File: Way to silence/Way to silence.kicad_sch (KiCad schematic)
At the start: 17 parts, among them J3 5V_Terminal, J4 Battery_Terminal, J5 LEDS Port, SW1 SW_SPDT, SW3 SW_SPST, U1 ESP32-WROOM-32-N16, U6 AMS1117CD-3.3

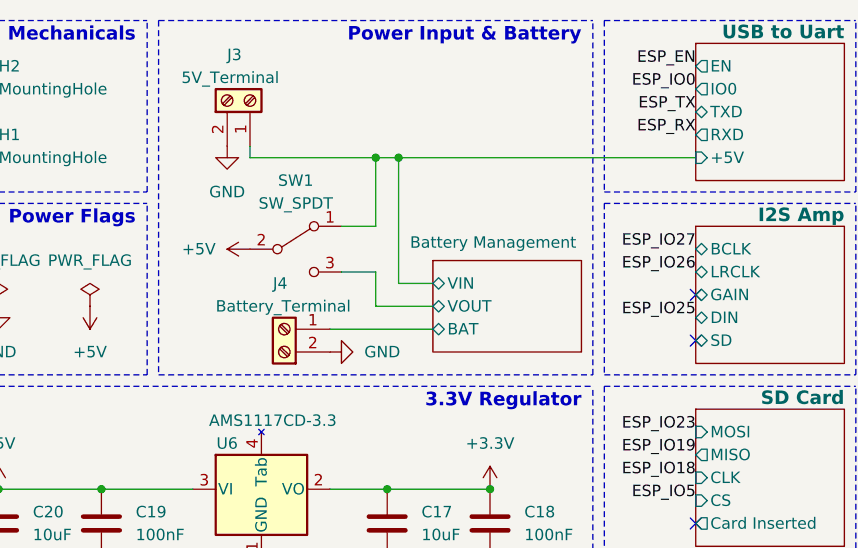
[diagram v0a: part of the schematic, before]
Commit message: [UDPT] Sheet name
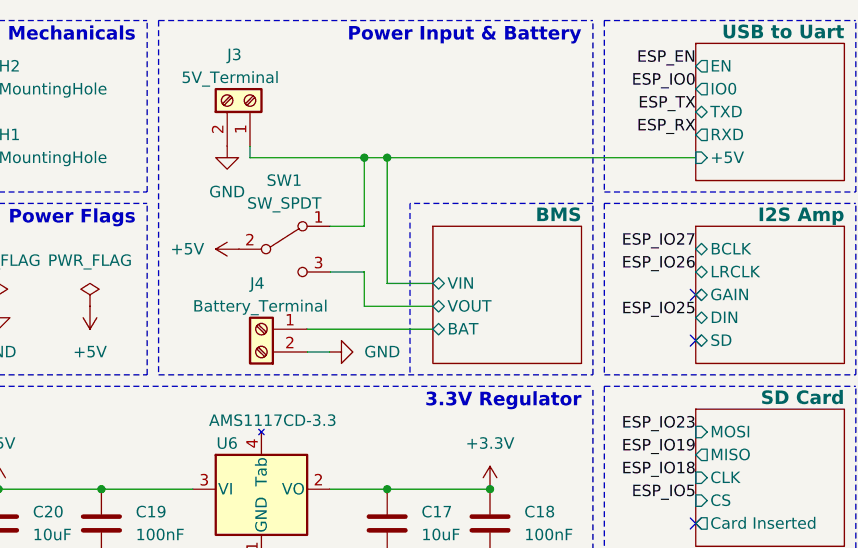
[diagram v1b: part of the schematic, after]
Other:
- sheet Battery Management renamed BMS
- moved on the sheet: J4, SW1
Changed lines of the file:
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@@
     (rev "1.0")
   )
-  (junction (at 144.78 30.48) (diameter 0) (color 0 0 0 0)
-  )
-  (junction (at 142.24 30.48) (diameter 0) (color 0 0 0 0)
-  )
   (junction (at 143.51 67.31) (diameter 0) (color 0 0 0 0)
   )
   (junction (at 100.33 67.31) (diameter 0) (color 0 0 0 0)
   )
+  (junction (at 143.51 30.48) (diameter 0) (color 0 0 0 0)
+  )
   (junction (at 111.76 67.31) (diameter 0) (color 0 0 0 0)
   )
   (junction (at 154.94 67.31) (diameter 0) (color 0 0 0 0)
+  )
+  (junction (at 140.97 30.48) (diameter 0) (color 0 0 0 0)
   )
   (junction (at 154.94 74.93) (diameter 0) (color 0 0 0 0)
@@
     (stroke (width 0) (type dash))
   )
-  (wire (pts (xy 148.59 46.99) (xy 142.24 46.99))
+  (wire (pts (xy 143.51 30.48) (xy 177.8 30.48))
+    (stroke (width 0) (type default))
+  )
+  (wire (pts (xy 148.59 46.99) (xy 140.97 46.99))
     (stroke (width 0) (type default))
   )
@@
     (stroke (width 0) (type dash))
   )
-  (wire (pts (xy 138.43 38.1) (xy 142.24 38.1))
+  (wire (pts (xy 137.16 38.1) (xy 140.97 38.1))
     (stroke (width 0) (type default))
   )
@@
     (stroke (width 0) (type dash))
   )
-  (wire (pts (xy 142.24 30.48) (xy 128.27 30.48))
+  (wire (pts (xy 140.97 30.48) (xy 143.51 30.48))
     (stroke (width 0) (type default))
   )
@@
     (stroke (width 0) (type dash))
   )
-  (wire (pts (xy 144.78 44.45) (xy 148.59 44.45))
+  (wire (pts (xy 143.51 44.45) (xy 148.59 44.45))
     (stroke (width 0) (type default))
   )
@@
     (stroke (width 0) (type dash))
   )
-  (wire (pts (xy 142.24 46.99) (xy 142.24 43.18))
+  (wire (pts (xy 140.97 46.99) (xy 140.97 43.18))
     (stroke (width 0) (type default))
   )
@@
     (stroke (width 0) (type dash))
   )
-  (wire (pts (xy 142.24 38.1) (xy 142.24 30.48))
+  (wire (pts (xy 140.97 38.1) (xy 140.97 30.48))
     (stroke (width 0) (type default))
   )
@@
     (stroke (width 0) (type dash))
   )
+  (polyline (pts (xy 166.37 35.56) (xy 146.05 35.56))
+    (stroke (width 0) (type dash))
+  )
   (wire (pts (xy 100.33 74.93) (xy 111.76 74.93))
     (stroke (width 0) (type default))
@@
     (stroke (width 0) (type dash))
   )
-  (wire (pts (xy 142.24 30.48) (xy 144.78 30.48))
-    (stroke (width 0) (type default))
-  )
   (polyline (pts (xy 60.96 15.24) (xy 60.96 34.29))
     (stroke (width 0) (type dash))
@@
     (stroke (width 0) (type dash))
   )
+  (wire (pts (xy 134.62 52.07) (xy 137.16 52.07))
+    (stroke (width 0) (type default))
+  )
   (polyline (pts (xy 167.64 74.93) (xy 195.58 74.93))
     (stroke (width 0) (type dash))
@@
     (stroke (width 0) (type dash))
   )
-  (wire (pts (xy 144.78 30.48) (xy 144.78 44.45))
+  (wire (pts (xy 143.51 30.48) (xy 143.51 44.45))
     (stroke (width 0) (type default))
   )
@@
     (stroke (width 0) (type dash))
   )
+  (polyline (pts (xy 146.05 35.56) (xy 146.05 54.61))
+    (stroke (width 0) (type dash))
+  )
   (polyline (pts (xy 195.58 74.93) (xy 195.58 55.88))
     (stroke (width 0) (type dash))
@@
     (stroke (width 0) (type dash))
   )
-  (wire (pts (xy 137.16 49.53) (xy 148.59 49.53))
+  (wire (pts (xy 134.62 49.53) (xy 148.59 49.53))
     (stroke (width 0) (type default))
   )
@@
     (stroke (width 0) (type default))
   )
+  (wire (pts (xy 140.97 30.48) (xy 128.27 30.48))
+    (stroke (width 0) (type default))
+  )
   (polyline (pts (xy 92.71 34.29) (xy 92.71 15.24))
     (stroke (width 0) (type dash))
@@
     (stroke (width 0) (type dash))
   )
-  (wire (pts (xy 144.78 30.48) (xy 177.8 30.48))
-    (stroke (width 0) (type default))
-  )
   (polyline (pts (xy 93.98 82.55) (xy 166.37 82.55))
     (stroke (width 0) (type dash))
@@
     (stroke (width 0) (type dash))
   )
-  (wire (pts (xy 142.24 43.18) (xy 138.43 43.18))
+  (wire (pts (xy 140.97 43.18) (xy 137.16 43.18))
     (stroke (width 0) (type default))
   )
@@
     )
   )
-  (symbol (lib_id "power:+5V") (at 128.27 40.64 90) (unit 1)
-    (in_bom yes) (on_board yes) (dnp no) (fields_autoplaced)
-    (property "Reference" "#PWR06" (at 132.08 40.64 0)
-      (effects (font (size 1.27 1.27)) hide)
-    )
-    (property "Value" "+5V" (at 124.46 40.64 90)
-      (effects (font (size 1.27 1.27)) (justify left))
-    )
-    (property "Footprint" "" (at 128.27 40.64 0)
-      (effects (font (size 1.27 1.27)) hide)
-    )
-    (property "Datasheet" "" (at 128.27 40.64 0)
+  (symbol (lib_id "power:+5V") (at 127 40.64 90) (unit 1)
+    (in_bom yes) (on_board yes) (dnp no) (fields_autoplaced)
+    (property "Reference" "#PWR06" (at 130.81 40.64 0)
+      (effects (font (size 1.27 1.27)) hide)
+    )
+    (property "Value" "+5V" (at 123.19 40.64 90)
+      (effects (font (size 1.27 1.27)) (justify left))
+    )
+    (property "Footprint" "" (at 127 40.64 0)
+      (effects (font (size 1.27 1.27)) hide)
+    )
+    (property "Datasheet" "" (at 127 40.64 0)
       (effects (font (size 1.27 1.27)) hide)
     )
@@
     )
   )
-  (symbol (lib_id "Way to silence:SW_SPDT") (at 133.35 40.64 0) (unit 1)
-    (in_bom yes) (on_board yes) (dnp no) (fields_autoplaced)
-    (property "Reference" "SW1" (at 133.35 33.02 0)
-      (effects (font (size 1.27 1.27)))
-    )
-    (property "Value" "SW_SPDT" (at 133.35 35.56 0)
-      (effects (font (size 1.27 1.27)))
-    )
-    (property "Footprint" "Way to silence:SW_SPDT" (at 132.08 26.67 0)
-      (effects (font (size 1.27 1.27)) hide)
-    )
-    (property "Datasheet" "~" (at 133.35 29.21 0)
-      (effects (font (size 1.27 1.27)) hide)
-    )
-    (property "LCSC" "C319013" (at 132.08 24.13 0)
+  (symbol (lib_id "Way to silence:SW_SPDT") (at 132.08 40.64 0) (unit 1)
+    (in_bom yes) (on_board yes) (dnp no) (fields_autoplaced)
+    (property "Reference" "SW1" (at 132.08 33.02 0)
+      (effects (font (size 1.27 1.27)))
+    )
+    (property "Value" "SW_SPDT" (at 132.08 35.56 0)
+      (effects (font (size 1.27 1.27)))
+    )
+    (property "Footprint" "Way to silence:SW_SPDT" (at 130.81 26.67 0)
+      (effects (font (size 1.27 1.27)) hide)
+    )
+    (property "Datasheet" "~" (at 132.08 29.21 0)
+      (effects (font (size 1.27 1.27)) hide)
+    )
+    (property "LCSC" "C319013" (at 130.81 24.13 0)
       (effects (font (size 1.27 1.27)) hide)
     )
@@
     )
   )
-  (symbol (lib_id "Way to silence:Screw_Terminal_01x02") (at 132.08 52.07 180) (unit 1)
+  (symbol (lib_id "Way to silence:Screw_Terminal_01x02") (at 129.54 52.07 180) (unit 1)
     (in_bom yes) (on_board yes) (dnp no)
-    (property "Reference" "J4" (at 130.81 44.45 0)
-      (effects (font (size 1.27 1.27)) (justify right))
-    )
-    (property "Value" "Battery_Terminal" (at 124.46 46.99 0)
-      (effects (font (size 1.27 1.27)) (justify right))
-    )
-    (property "Footprint" "Way to silence:Screw_Terminal_3.5" (at 132.08 52.07 0)
-      (effects (font (size 1.27 1.27)) hide)
-    )
-    (property "Datasheet" "~" (at 132.08 52.07 0)
-      (effects (font (size 1.27 1.27)) hide)
-    )
-    (property "LCSC" "C784942" (at 132.08 58.42 0)
+    (property "Reference" "J4" (at 128.27 44.45 0)
+      (effects (font (size 1.27 1.27)) (justify right))
+    )
+    (property "Value" "Battery_Terminal" (at 121.92 46.99 0)
+      (effects (font (size 1.27 1.27)) (justify right))
+    )
+    (property "Footprint" "Way to silence:Screw_Terminal_3.5" (at 129.54 52.07 0)
+      (effects (font (size 1.27 1.27)) hide)
+    )
+    (property "Datasheet" "~" (at 129.54 52.07 0)
+      (effects (font (size 1.27 1.27)) hide)
+    )
+    (property "LCSC" "C784942" (at 129.54 58.42 0)
       (effects (font (size 1.27 1.27)) hide)
     )
@@
     )
   )
-  (sheet (at 148.59 41.91) (size 16.51 10.16)
+  (sheet (at 148.59 38.1) (size 16.51 15.24)
     (stroke (width 0.1524) (type solid))
     (fill (color 0 0 0 0.0000))
-    (property "Sheetname" "Battery Management" (at 146.05 40.64 0)
-      (effects (font (size 1.27 1.27)) (justify left bottom))
-    )
-    (property "Sheetfile" "battery_management.kicad_sch" (at 148.59 52.6546 0)
+    (property "Sheetname" "BMS" (at 165.1 36.83 0)
+      (effects (font (size 1.5 1.5) bold) (justify right))
+    )
+    (property "Sheetfile" "battery_management.kicad_sch" (at 148.59 48.8446 0)
       (effects (font (size 1.27 1.27)) (justify left top) hide)
     )
